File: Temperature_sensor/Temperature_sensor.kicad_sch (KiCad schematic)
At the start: 11 parts, among them IC1 TC7660, U1 TP4056, U2 ESP32-S3-ZERO

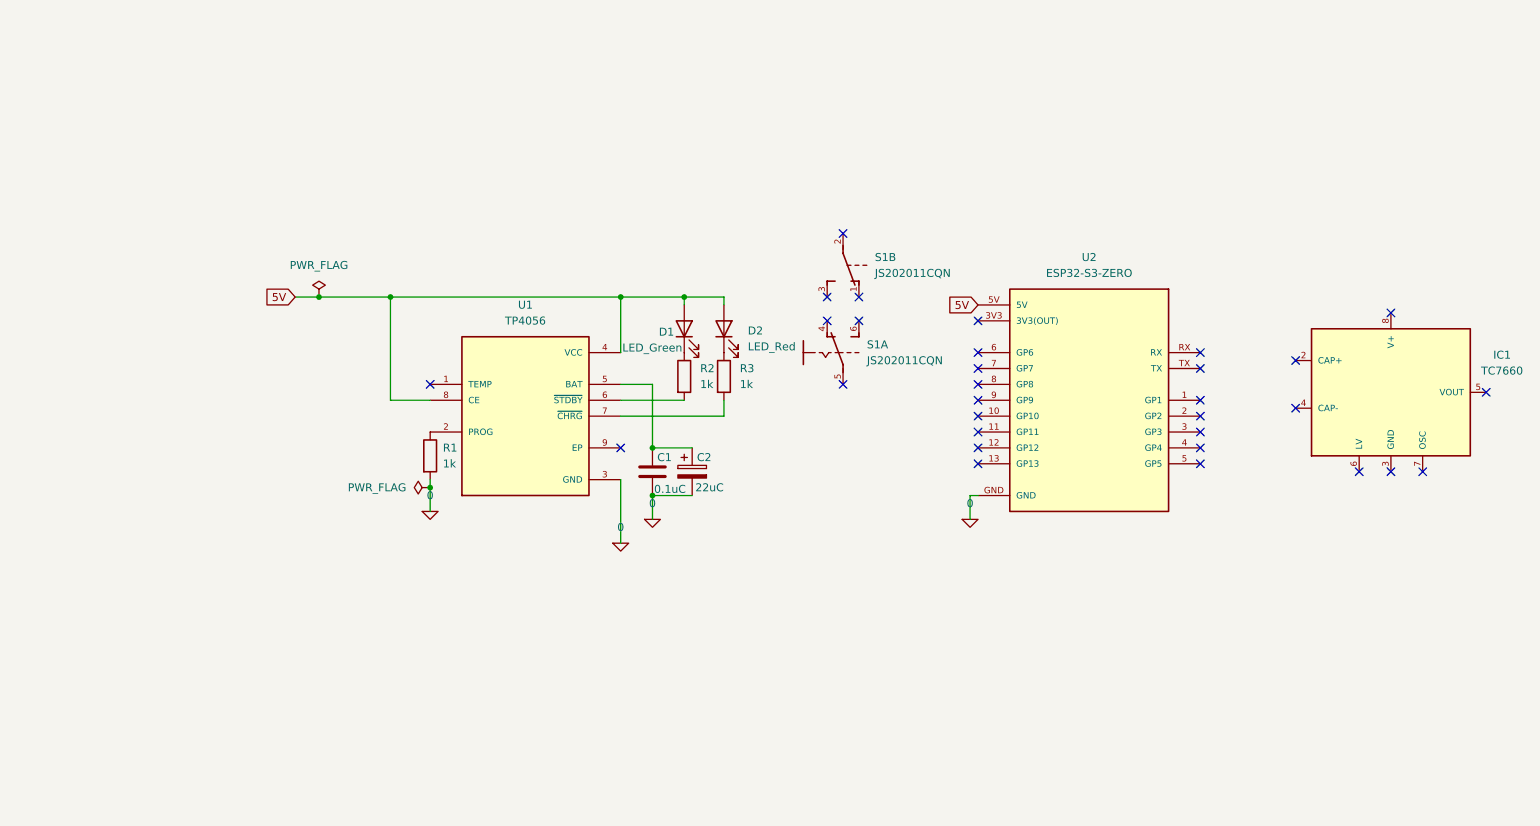
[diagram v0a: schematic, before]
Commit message: final
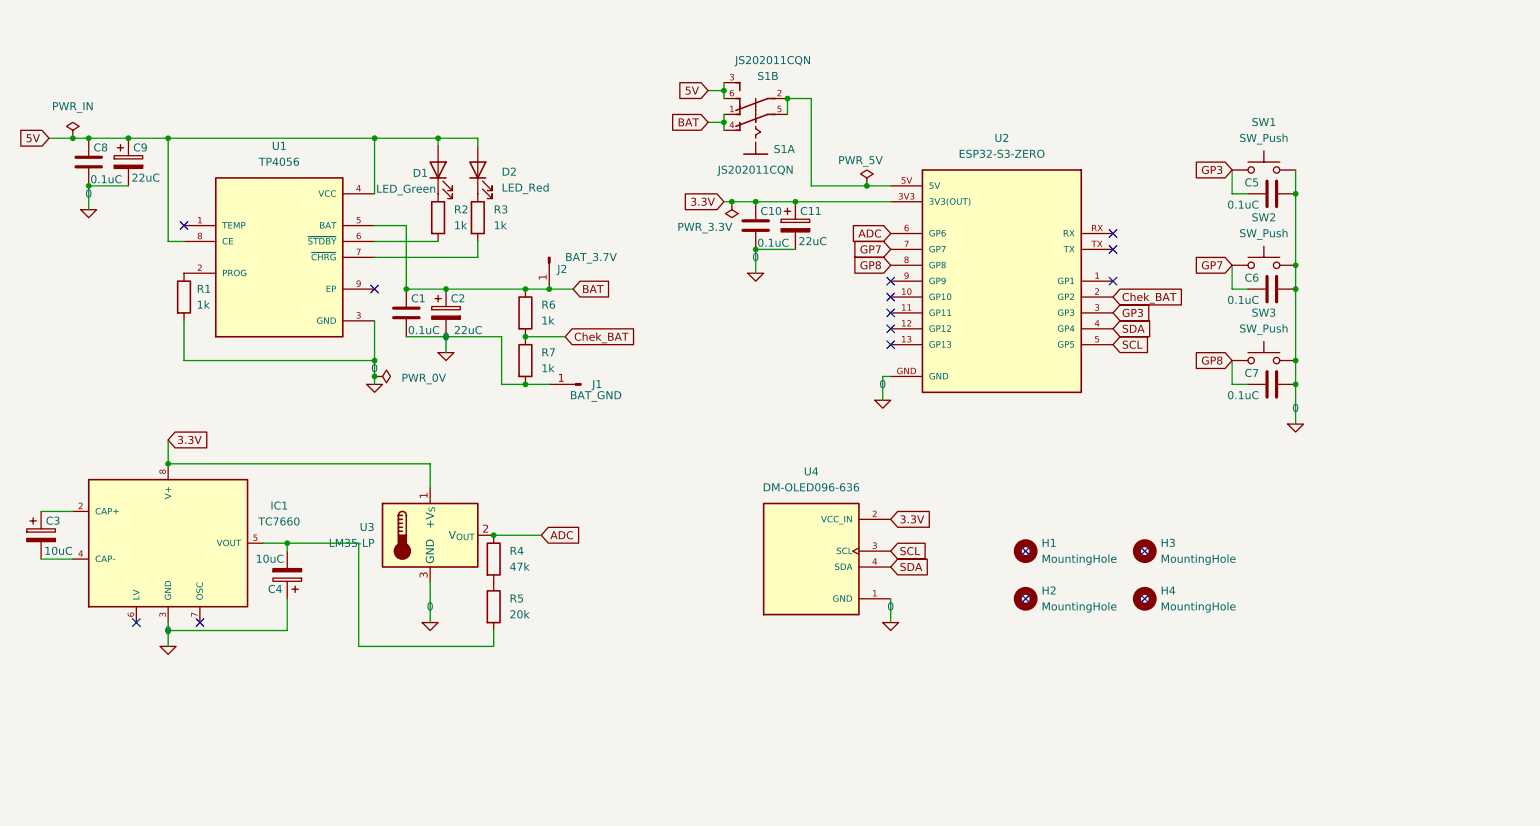
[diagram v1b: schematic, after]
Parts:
- added C10, C5, C6, C7, C8: 0.1uC, Capacitor_SMD:C_0805_2012Metric, symbol Device:C
- added C11, C9: 22uC, Capacitor_THT:CP_Radial_D5.0mm_P2.00mm, symbol Device:C_Polarized
- added C3, C4: 10uC, Capacitor_THT:CP_Radial_D5.0mm_P2.00mm, symbol Device:C_Polarized
- added H1, H2, H3, H4: MountingHole, MountingHole:MountingHole_3.2mm_M3, symbol Mechanical:MountingHole
- added J1: BAT_GND, Connector_PinSocket_2.00mm:PinSocket_1x01_P2.00mm_Vertical, symbol Connector:Conn_01x01_Pin
- added J2: BAT_3.7V, Connector_PinSocket_2.00mm:PinSocket_1x01_P2.00mm_Vertical, symbol Connector:Conn_01x01_Pin
- added R4: 47k, Resistor_THT:R_Axial_DIN0207_L6.3mm_D2.5mm_P10.16mm_Horizontal, symbol Device:R
- added R5: 20k, Resistor_THT:R_Axial_DIN0207_L6.3mm_D2.5mm_P10.16mm_Horizontal, symbol Device:R
- added R6, R7: 1k, LED_SMD:LED_0603_1608Metric_Pad1.05x0.95mm_HandSolder, symbol Device:R
- added SW1, SW2, SW3: SW_Push, SW_Push:SW_TH_Tactile_Omron_B3F-10xx, symbol Switch:SW_Push
- added U3: LM35-LP, Package_TO_SOT_THT:TO-92, symbol Sensor_Temperature:LM35-LP
- added U4: DM-OLED096-636, OLED:MODULE_DM-OLED096-636, symbol OLED:DM-OLED096-636
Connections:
- net 0: now also IC1.3 (GND), C10.2, C11.2, C4.1, C5.2, C6.2, C7.2, C8.2, C9.2, J1.1 (Pin_1), R7.2, SW1.2, SW2.2, SW3.2, U3.3 (GND), U4.1 (GND)
- net 5V: now also S1.3, S1.6, C8.1, C9.1; no longer U2.5V
- net Chek_BAT: now reaches U2.2 (GP2)
- net Chek_BAT: now also R6.2, R7.1
- net GP3: now reaches U2.3 (GP3)
- net GP3: now also C5.1, SW1.1
- net 3.3V: now reaches U2.3V3 (3V3(OUT))
- net 3.3V: now also IC1.8 (V+), C10.1, C11.1, U3.1 (+V_{S}), U4.2 (VCC_IN)
- net SDA: now reaches U2.4 (GP4)
- net SDA: now also U4.4 (SDA)
- net SCL: now reaches U2.5 (GP5)
- net SCL: now also U4.3 (SCL)
- net ADC: now reaches U2.6 (GP6)
- net ADC: now also R4.1, U3.2 (V_{OUT})
- net GP7: now reaches U2.7 (GP7)
- net GP7: now also C6.1, SW2.1
- net GP8: now reaches U2.8 (GP8)
- net GP8: now also C7.1, SW3.1
- net BAT: now reaches C1.1, C2.1, U1.5 (BAT)
- net BAT: now also S1.1, S1.4, J2.1 (Pin_1), R6.1
- net at S1.2: now also S1.5, U2.5V
- net at IC1.2 (CAP+): now also C3.1
- net at IC1.4 (CAP-): now also C3.2
- net at IC1.5 (VOUT): now also C4.2, R5.2
- new net: R4.2, R5.1
- no-connect marks 31 -> 16
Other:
- moved on the sheet: C1, C2, D1, D2, IC1, R1, R2, R3, S1A, S1B, U1, U2

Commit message: final
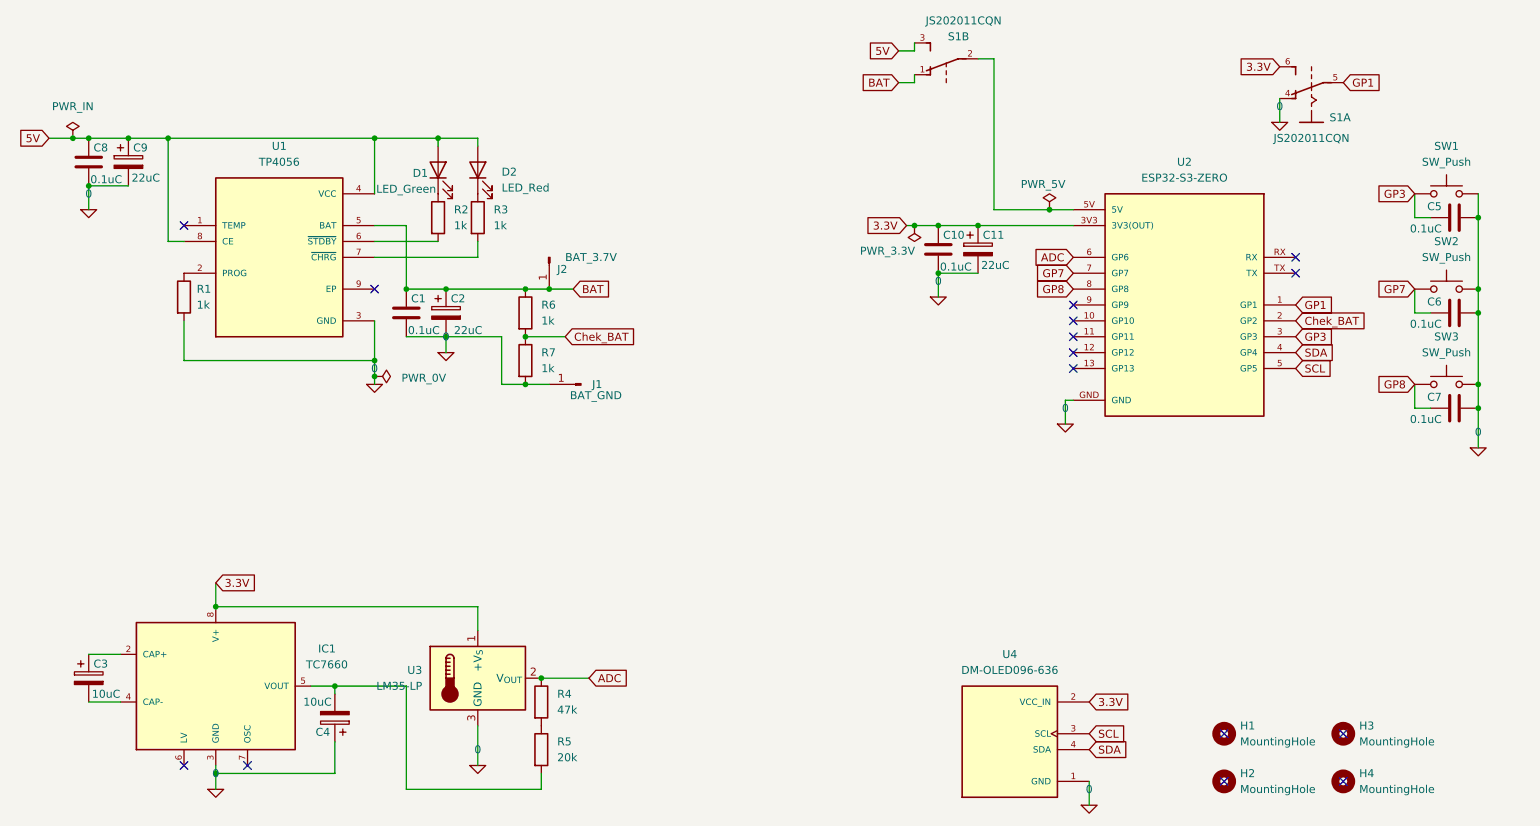
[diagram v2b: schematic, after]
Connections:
- net 0: now also S1.4
- net 3.3V: now also S1.6
- net 5V: no longer S1.6
- net BAT: no longer S1.4
- net GP1: now reaches U2.1 (GP1)
- net GP1: now also S1.5
- net at S1.2, U2.5V: no longer S1.5
- no-connect marks 16 -> 15
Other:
- moved on the sheet: C10, C11, C3, C4, C5, C6, C7, H1, H2, H3, H4, IC1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
